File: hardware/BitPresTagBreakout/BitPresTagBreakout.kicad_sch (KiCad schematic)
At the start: 10 parts, among them J3 Conn_01x17, J4 Conn_01x17, U2 AT25XE321, U3 LPS27HHWTR, U4 adxl362

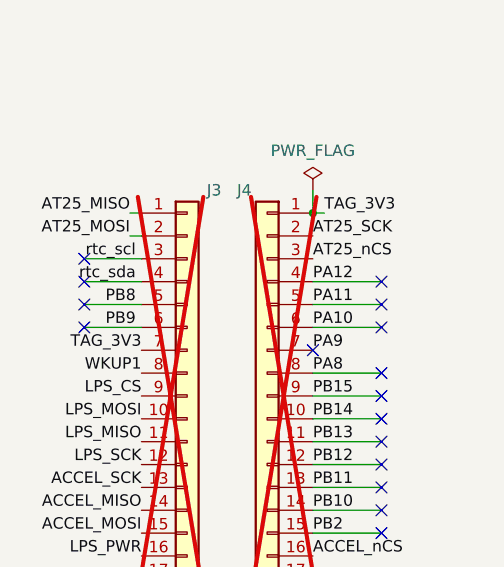
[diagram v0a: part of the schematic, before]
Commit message: update proto boards
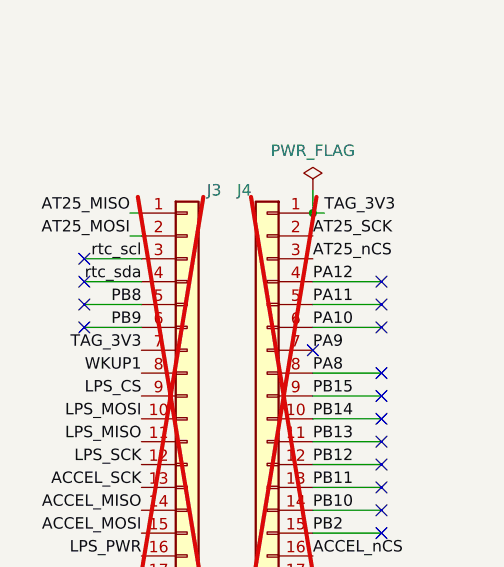
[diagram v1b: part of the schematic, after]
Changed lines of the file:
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@@
 	)
 	(label "rtc_sda"
-		(at 37.465 64.77 180)
+		(at 38.1 64.77 180)
 		(effects
 			(font
@@
 	)
 	(label "rtc_scl"
-		(at 37.465 62.23 180)
+		(at 38.1 62.23 180)
 		(effects
 			(font
@@
 	)
 	(label "PB8"
-		(at 37.465 67.31 180)
+		(at 38.1 67.31 180)
 		(effects
 			(font
@@
 	)
 	(label "PB9"
-		(at 37.465 69.85 180)
-		(effects
-			(font
+		(at 38.1 69.85 180)
+		(effects
+			(font
